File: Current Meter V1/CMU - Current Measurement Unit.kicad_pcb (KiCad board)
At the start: 4 copper layers, 94.5 x 119.5 mm, 28 parts, among them J401 I2C OLED Display Connector, J501 Connector, U201 MCP6002-xSN

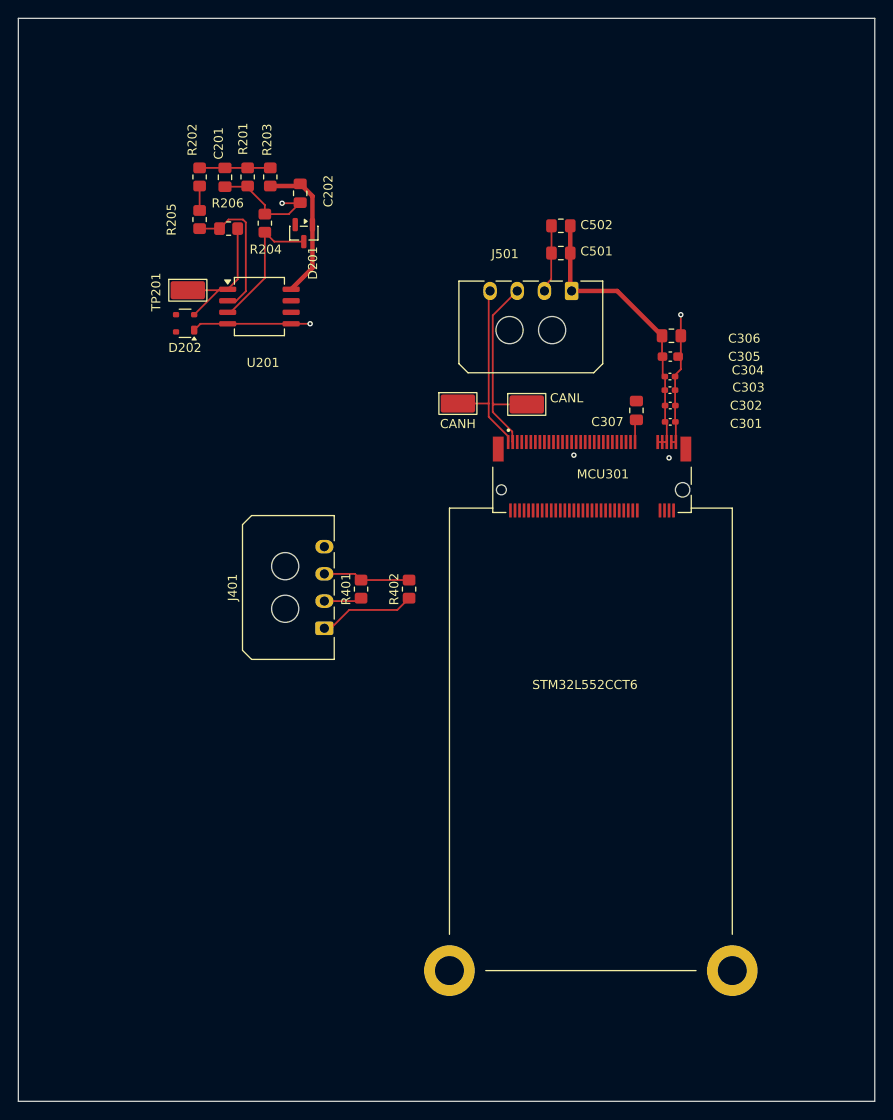
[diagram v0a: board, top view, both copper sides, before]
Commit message: layup updated
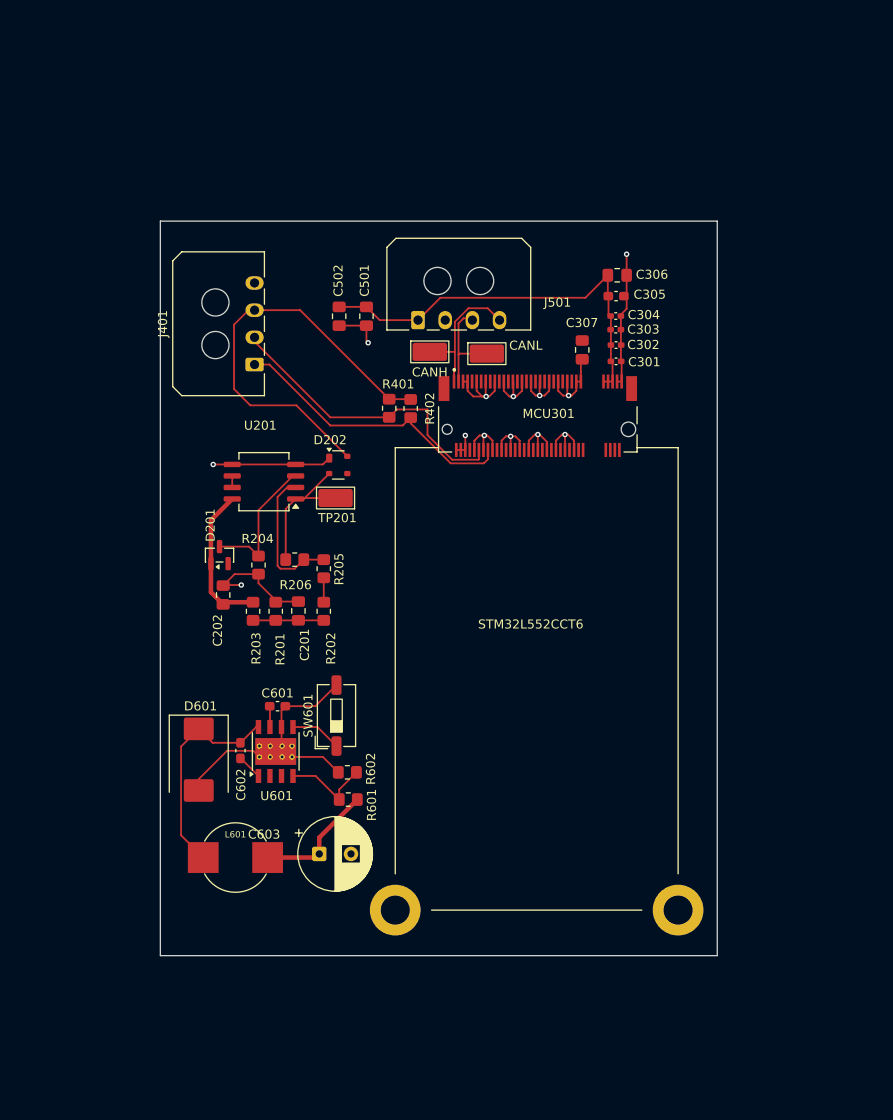
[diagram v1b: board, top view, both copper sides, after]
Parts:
- added C601: 10u, Capacitor_SMD:C_0603_1608Metric_Pad1.08x0.95mm_HandSolder, F.Cu at (131.5, 117.9)
- added C602: 10n, Capacitor_SMD:C_0603_1608Metric_Pad1.08x0.95mm_HandSolder, F.Cu at (127.4, 122.8)
- added C603: 220u, Capacitor_THT:CP_Radial_D8.0mm_P3.50mm, F.Cu at (136.1, 134.2)
- added D601: B340, Diode_SMD:D_SMC, F.Cu at (122.8, 123.8)
- added L601: 15u, bfr_inductors:CDRH104RNP-150NC, F.Cu at (126.9, 134.6)
- added R601: 10k, Resistor_SMD:R_0805_2012Metric_Pad1.20x1.40mm_HandSolder, F.Cu at (139.3, 128.2)
- added R602: 3.3k, Resistor_SMD:R_0805_2012Metric_Pad1.20x1.40mm_HandSolder, F.Cu at (139.2, 125.2)
- added SW601: SW_DIP_x01, Button_Switch_SMD:SW_DIP_SPSTx01_Slide_6.7x4.1mm_W6.73mm_P2.54mm_LowProfile_JPin, F.Cu at (138.0, 118.9)
- added U601: TPS5430DDAR, Package_SO:TI_SO-PowerPAD-8_ThermalVias, F.Cu at (131.3, 122.9)
- moved R202 49.8 mm to (136.6, 107.4), turned to -90 degrees
- moved C201 48.5 mm to (133.8, 107.4), turned to -90 degrees
- moved R201 48.0 mm to (131.3, 107.4), turned to -90 degrees
- moved R203 48.0 mm to (128.8, 107.4), turned to 90 degrees
- moved C202 45.1 mm to (125.5, 105.6), turned to 90 degrees
- moved R205 40.9 mm to (136.6, 102.7), turned to 90 degrees
- moved R204 37.7 mm to (129.4, 102.3), turned to 90 degrees
- moved R206 37.3 mm to (133.4, 101.7), turned to 180 degrees
- moved D201 36.7 mm to (125.1, 101.2), turned to 90 degrees
- moved J401 30.1 mm to (129.0, 80.2)
- moved TP201 28.1 mm to (137.9, 94.9), turned to 180 degrees
- moved C502 26.4 mm to (138.3, 74.9), turned to -90 degrees
- moved D202 23.0 mm to (138.2, 91.3), turned to 0 degrees
- moved C501 22.6 mm to (141.3, 74.9), turned to -90 degrees
- moved R401 20.2 mm to (143.8, 85.0)
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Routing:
- net GND: track 50.8 -> 131.1 mm, vias 5 -> 13
- net +3V3: track 9.63 -> 46.9 mm
- net /display/I2C_SCL: track 4.18 -> 34.4 mm
- net /buck/SW_NODE: track 0.00 -> 24.0 mm
- net /display/I2C_SDA: track 10.7 -> 32.6 mm
- net /buck/+5_V: track 0.00 -> 13.6 mm
- net /connector/+5_V: track 32.2 -> 45.5 mm
- net /connector/CAN-: track 22.5 -> 11.4 mm
- net Net-(U601-VSENSE): track 0.00 -> 9.96 mm
- net Net-(U601-EN): track 0.00 -> 5.67 mm
- net /connector/CAN+: track 21.0 -> 15.5 mm
- net Net-(U601-BOOT): track 0.00 -> 2.79 mm
- net /buck/VIN: track 0.00 -> 2.31 mm
- net Net-(U201B--): track 0.00 -> 1.27 mm
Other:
- board size 94.5 x 119.5 mm -> 61.5 x 81.1 mm
